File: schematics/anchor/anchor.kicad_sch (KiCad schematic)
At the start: 38 parts, among them J1 IEC_60320_C14_Receptacle, J16 Screw_Terminal_01x01, J18 Screw_Terminal_01x01, J2 120VAC-L, J3 120VAC-N, J4 Earth, M26 Fan, M27 Fan, M3 Fan, M4 Fan, SW1 SW_DPST, SW3 SW_SPST_NC_Temperature, SW5 Thermostat, T1 Meanwell_UHP-200-48, T2 Meanwell_UHP-200-24, T3 Meanwell_UHP-200-5, U1 Crydom_D2440_SPST_SSR-NO, U2 Crydom_D2440_SPST_SSR-NO, U3 Crydom_D2440_SPST_SSR-NO, U4 Schneider_Electric_DPE25BL, U5 Crydom_D2440_SPST_SSR-NO

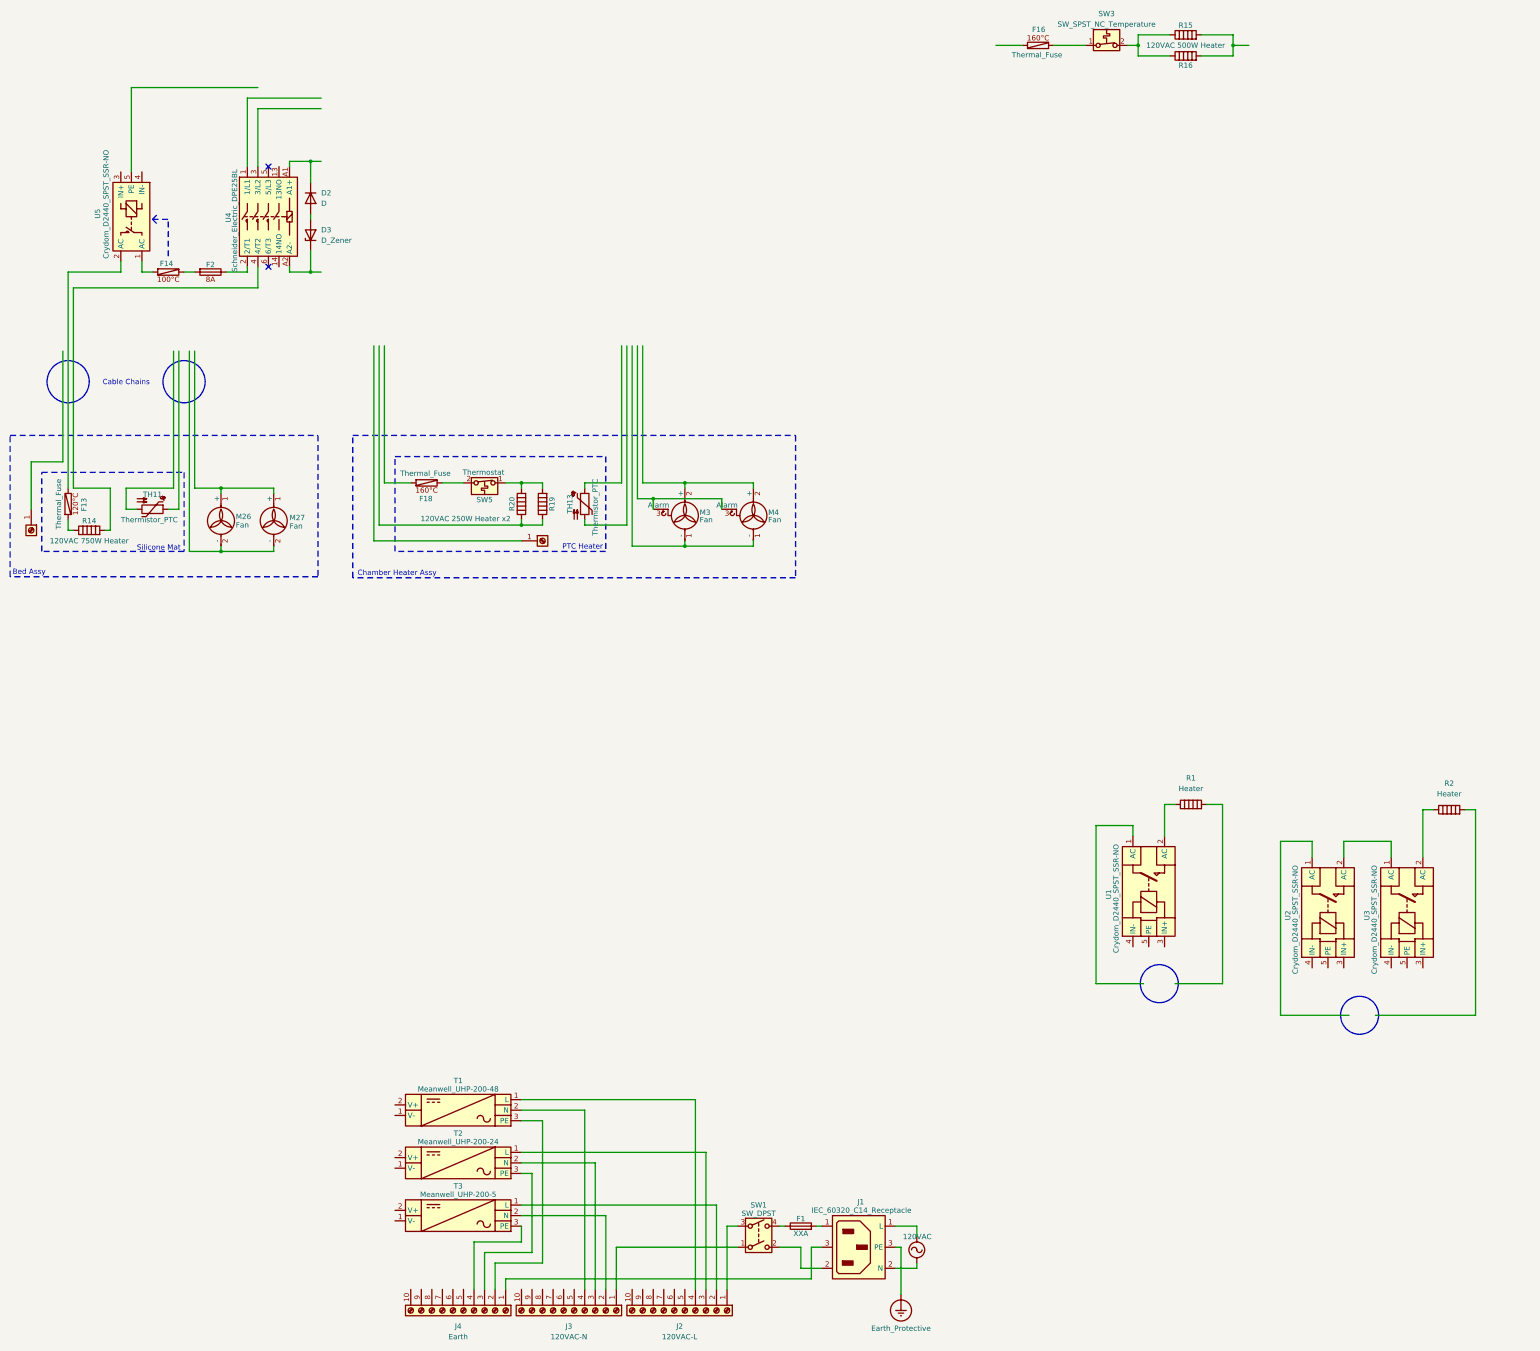
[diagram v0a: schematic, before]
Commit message: Start DFMEA study
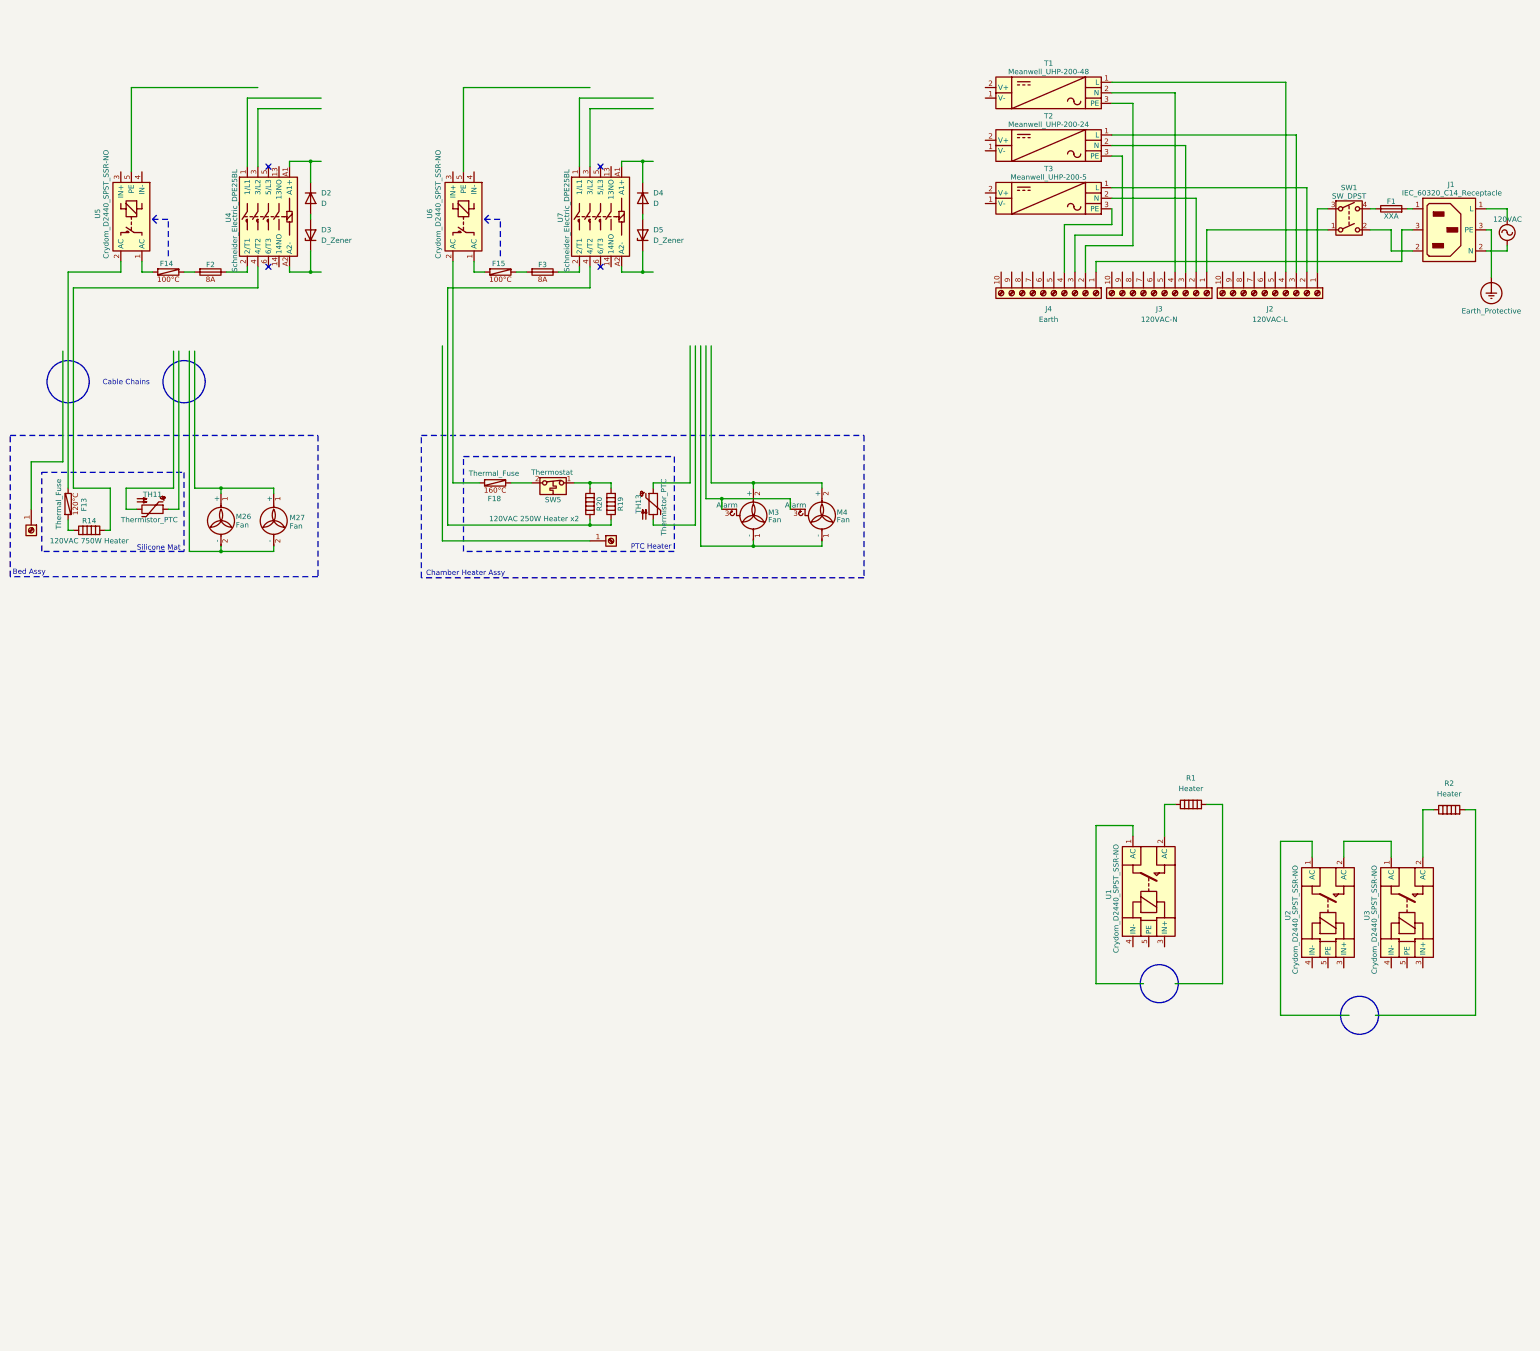
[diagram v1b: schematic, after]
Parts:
- removed F16: Thermal_Fuse, symbol jmatt:Thermal_Fuse
- removed R15, R16: 120VAC 500W Heater, symbol Device:Heater
- removed SW3: SW_SPST_NC_Temperature, symbol jmatt:SW_SPST_NC_Temperature
- added D4: D, symbol Device:D
- added D5: D_Zener, symbol Device:D_Zener
- added F15: Thermal_Fuse, symbol jmatt:Thermal_Fuse
- added F3: Fuse, symbol Device:Fuse
- added U6: Crydom_D2440_SPST_SSR-NO, symbol jmatt:Crydom_D2440_SPST_SSR-NO
- added U7: Schneider_Electric_DPE25BL, symbol jmatt:Schneider_Electric_DPE25BL
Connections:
- net at F18.2: now also U6.2 (AC)
- net at R19.1, R20.1: now also U7.4 (4/T2)
- net at J1.1 (L): now also F1.2
- new net: D5.1 (K), U7.A2 (A2-)
- new net: D4.2 (A), D5.2 (A)
- new net: F3.1, U7.2 (2/T1)
- new net: D4.1 (K), U7.A1 (A1+)
- new net: F15.2, U6.1 (AC)
- new net: F15.1, F3.2
- no-connect marks 2 -> 4
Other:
- company: (none) -> jmatt
- title: (none) -> Anchor
- moved on the sheet: F1, F18, J1, J2, J3, J4, M3, M4, R19, R20, SW1, SW5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
